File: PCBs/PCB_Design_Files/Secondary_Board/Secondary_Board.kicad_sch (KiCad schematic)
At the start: 6 parts, among them J1 Conn_FFC_8pin, J2 Conn_01x08_Pin

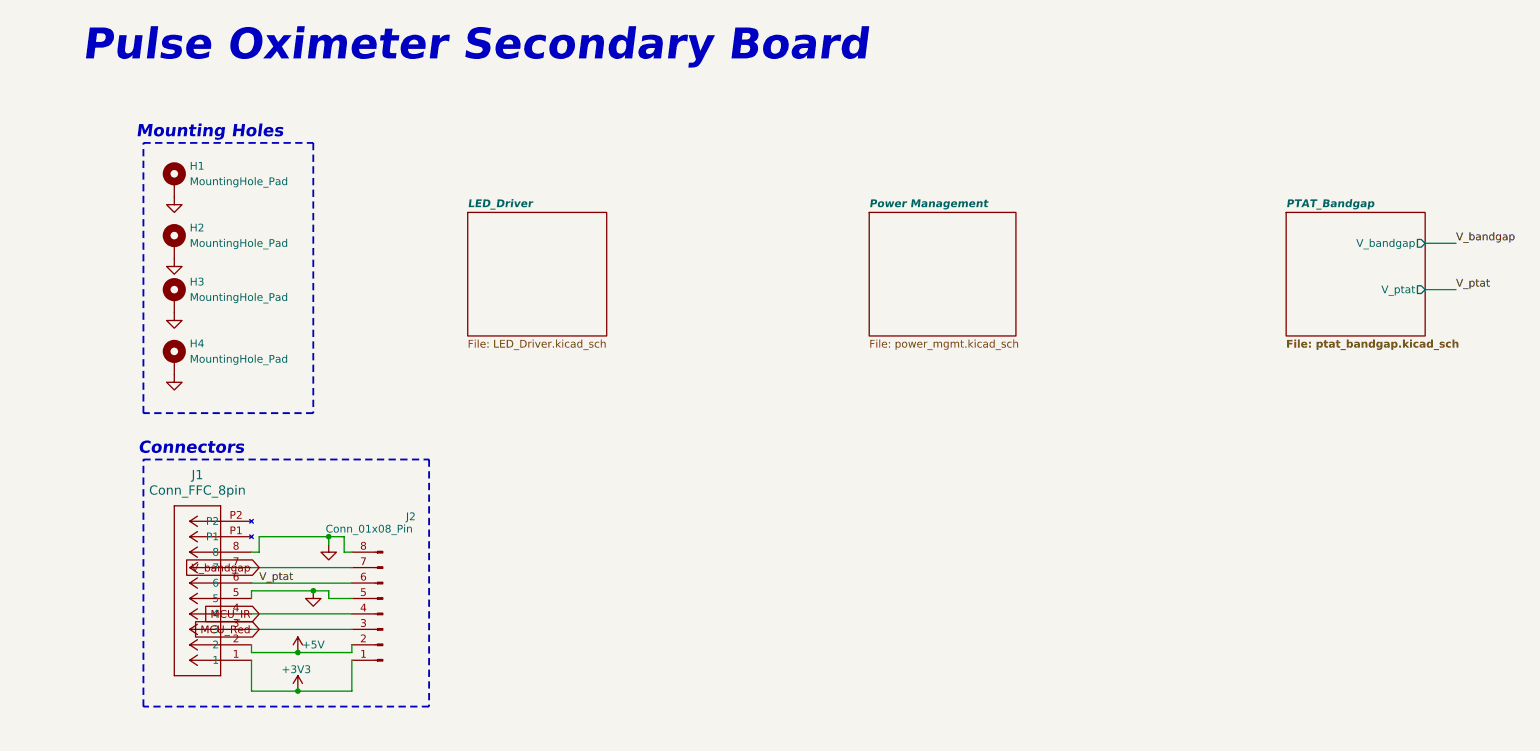
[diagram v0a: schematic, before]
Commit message: secondary board connectors
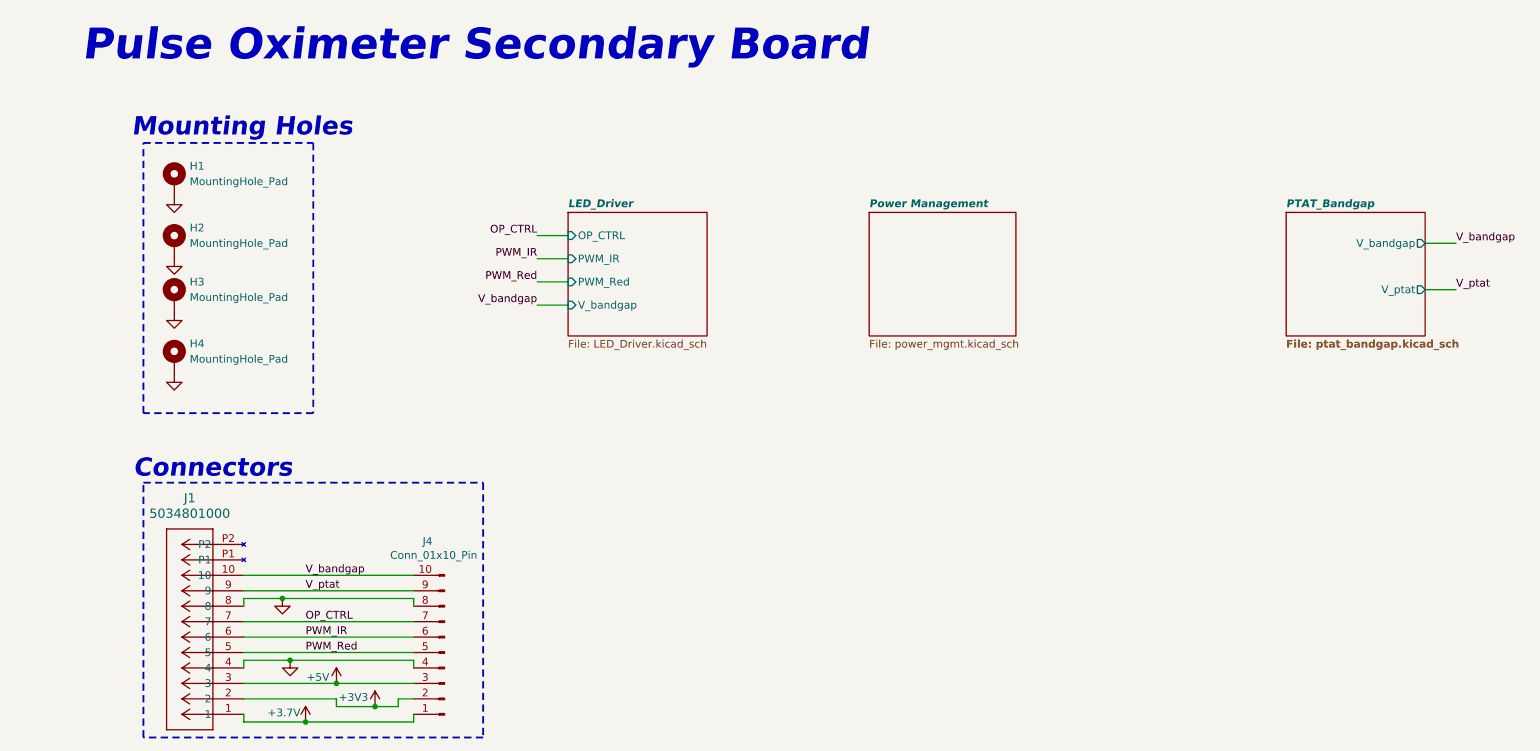
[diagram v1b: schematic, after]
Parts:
- removed J1: Conn_FFC_8pin, Project Footprints:Conn_FFC_8pin, symbol Project_Symbols:Conn_FFC_8pin
- removed J2: Conn_01x08_Pin, Connector_PinHeader_2.54mm:PinHeader_1x08_P2.54mm_Vertical, symbol Connector:Conn_01x08_Pin
- added J1: 5034801000, Project Footprints:Conn_FFC_10pin, symbol Project_Symbols:5034801000
- added J4: Conn_01x10_Pin, Connector_PinHeader_2.54mm:PinHeader_1x10_P2.54mm_Vertical, symbol Connector:Conn_01x10_Pin
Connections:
- net +3V3: now also J1.2, J4.2 (Pin_2)
- net +5V: now also J1.3, J4.3 (Pin_3)
- net GND: now also J1.4, J1.8, J4.4 (Pin_4), J4.8 (Pin_8)
- net V_bandgap: now also J1.10, J4.10 (Pin_10)
- net V_ptat: now also J1.9, J4.9 (Pin_9)
- new net +3.7V: J1.1, J4.1 (Pin_1)
- new net OP_CTRL: J1.7, J4.7 (Pin_7)
- new net PWM_IR: J1.6, J4.6 (Pin_6)
- new net PWM_Red: J1.5, J4.5 (Pin_5)
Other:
- sheet LED_Driver ports: added OP_CTRL, PWM_IR, PWM_Red, V_bandgap; removed none
